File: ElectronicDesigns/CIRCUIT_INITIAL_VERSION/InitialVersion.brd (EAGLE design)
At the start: 100 x 80 mm, 7 parts, among them U1 TLV1117-18IDCYG3

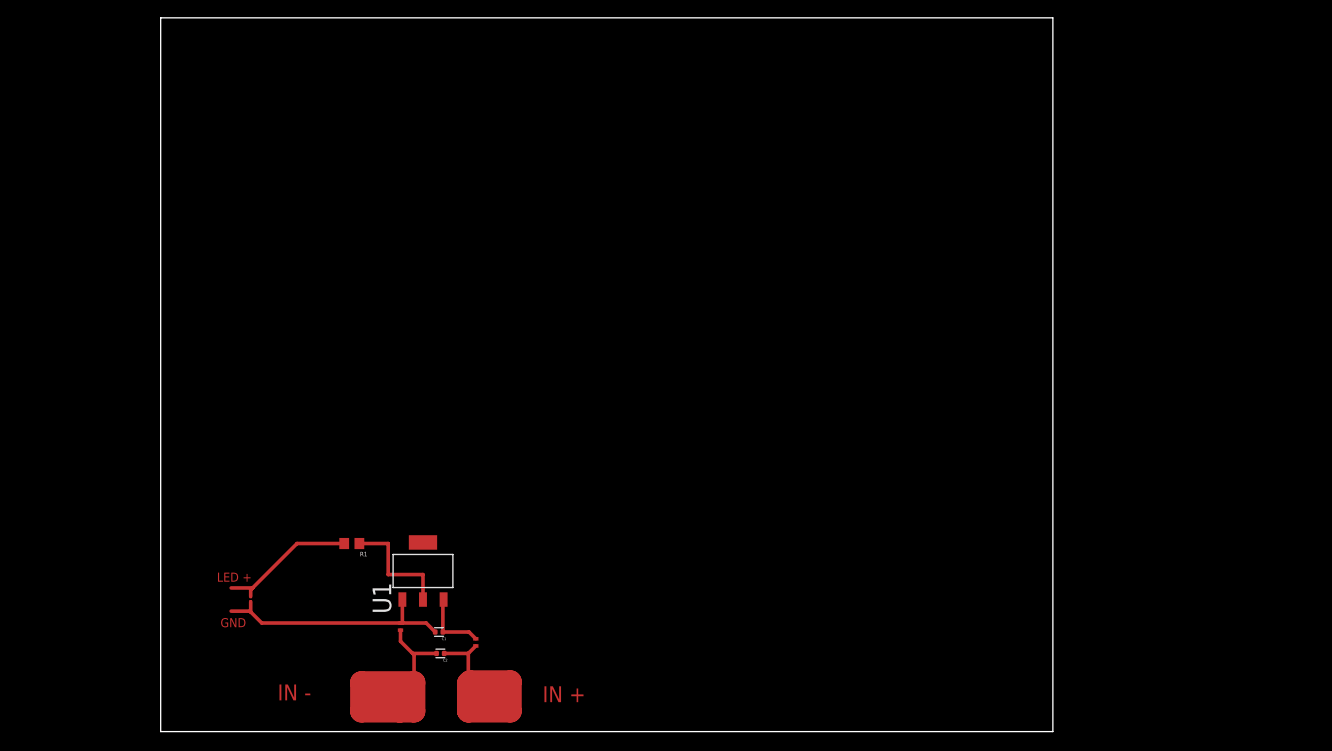
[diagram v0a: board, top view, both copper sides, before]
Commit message: Initial Circuit Version
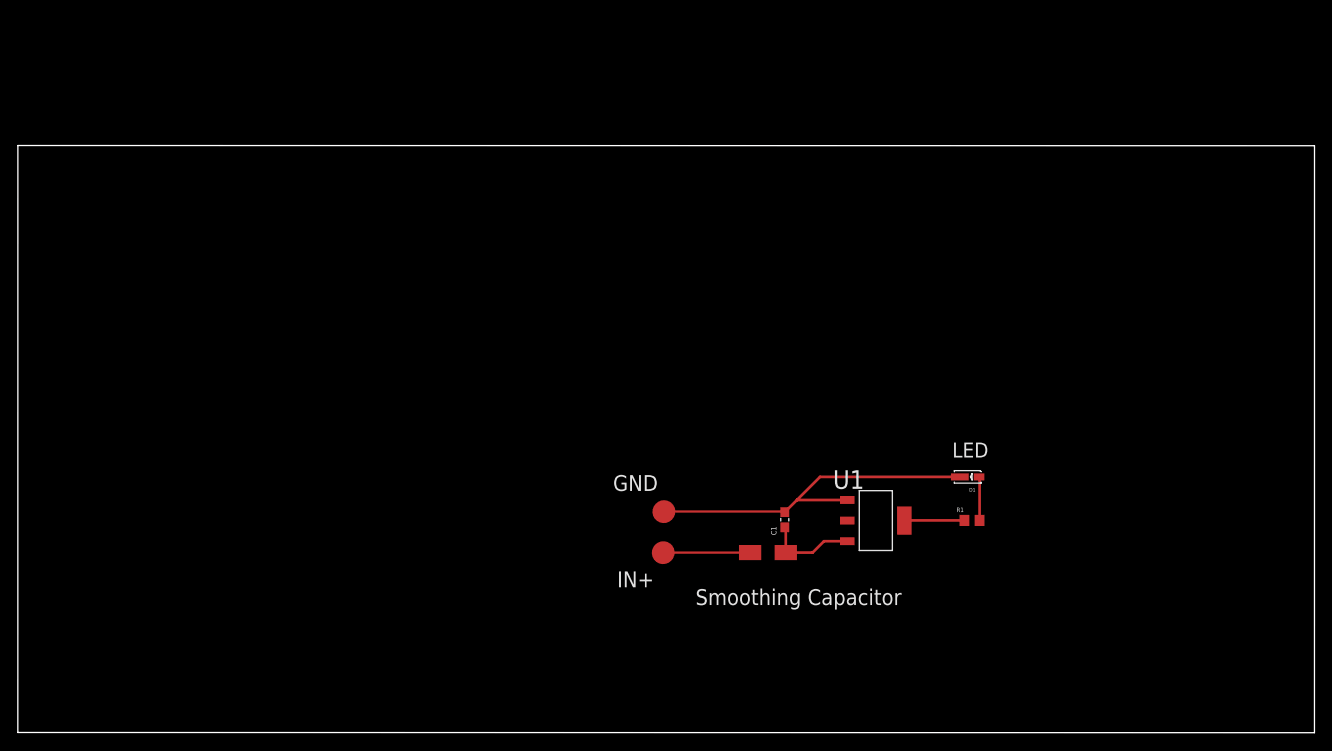
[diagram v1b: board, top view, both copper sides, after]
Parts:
- removed C2: AMK105BJ225MV-F, AMK105BJ225MV-F:CAPC1005X55N
- removed U$2, U$3: SCHOTTKY0402, Schottki_0402:0402_MURATA
- removed U$4: CREE-TR2227, CREE-TR2227:CREE-TR2227
- added D1: WL-SWTP3014, WL-SWTP:WL-SWTP_3014
- added U$1: B220A-13-F, Schottky_0603:SMA-DIODE
- C1: value AMK105BJ225MV-F -> 06036D225KAT2A; device AMK105BJ225MV-F:CAPC1005X55N -> Capacitor_2.2uF_0603:CAPC1608X90
- moved R1 69.6 mm to (90.9, 23.7), turned to 0 degrees
- moved U1 51.1 mm to (80.2, 23.6), turned to 0 degrees
- moved C1 40.7 mm to (70.0, 23.8), turned to 90 degrees
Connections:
- removed net IN-: C2.2, U$3.P$2
- net GND: now also D1.1; no longer U$3.P$1, U$4.P$2
- net IN+: now also U$1.1; no longer C2.1, U$2.P$1
- net N$1: now also U1.4; no longer U1.2
- net N$2: now also D1.2; no longer U$4.P$1
- net N$4: now also U$1.2; no longer U$2.P$2
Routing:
- net IN-: track 32.2 -> 0.00 mm
- net IN+: track 26.5 -> 9.76 mm
- net GND: track 27.6 -> 40.5 mm
- net N$2: track 15.8 -> 4.90 mm
- net N$1: track 13.4 -> 6.74 mm
- net N$4: track 7.68 -> 10.3 mm
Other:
- board size 100 x 80 mm -> 145.3 x 65.8 mm
- board text added: "IN+"
- board text added: "LED"
- board text added: "Smoothing Capacitor"
- board text removed: "IN +"
- board text removed: "IN -"
- board text removed: "LED +"
